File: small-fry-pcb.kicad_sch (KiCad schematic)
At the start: 139 parts, among them U1 Pico

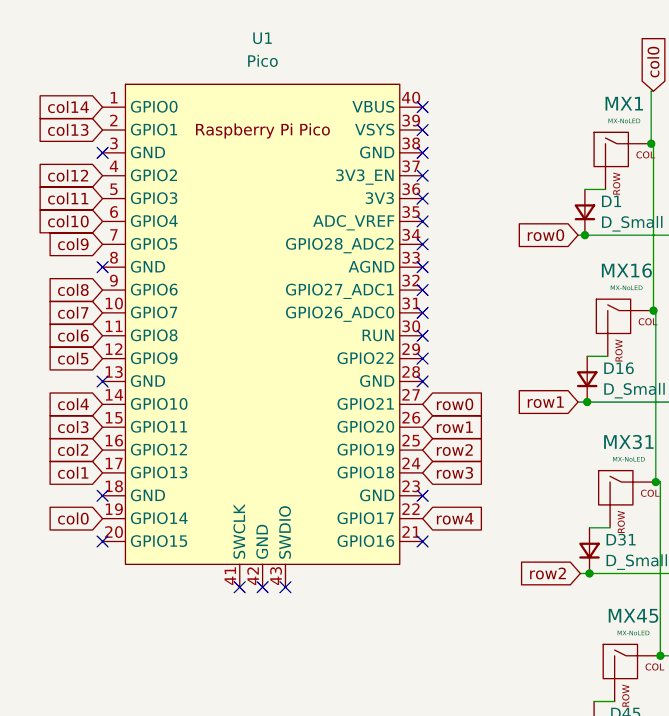
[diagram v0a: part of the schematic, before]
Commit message: Squashed commit of the following:
commit e493926800ae8eeeb9c8551a418d401659cc4f4a
Author: anchovie-codes <littlebrother.free@gmail.com>
Date:   Sun Nov 10 19:39:24 2024 -0500

    updated edge cuts and gerbers

commit a852bf54e9e750d94bc40db8a16316f7cdac5ac1
Author: anchovie-codes <littlebrother.free@gmail.com>
Date:   Sat Sep 28 17:49:30 2024 -0400

    fixed rows, generated gerbers

commit 9d77bf2fb49dd0b8cbfb8cfda25d822d23244967
Author: anchovie-codes <littlebrother.free@gmail.com>
Date:   Sat Sep 28 13:01:13 2024 -0400

    fixed cols

commit 5f5487953ddbebd1258b34876b9f208a7da505d8
Author: anchovie-codes <littlebrother.free@gmail.com>
Date:   Fri Sep 27 21:14:36 2024 -0400

    made it a fish
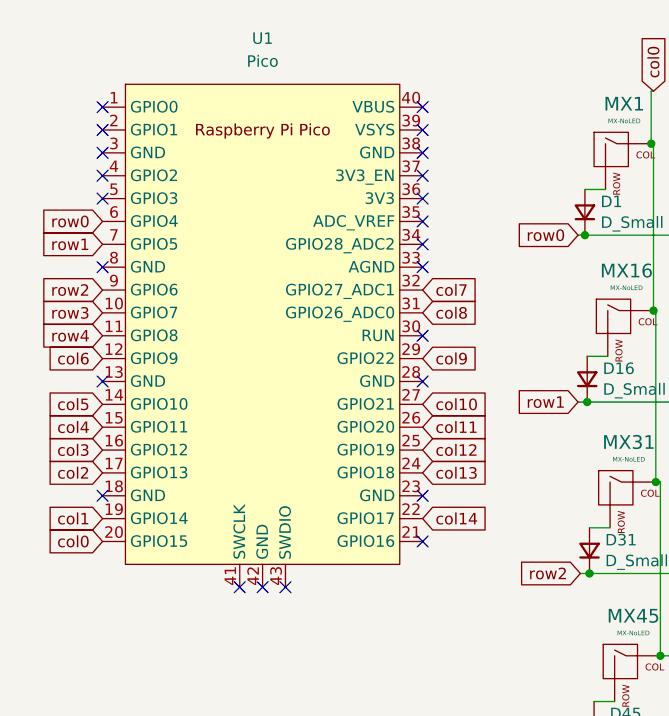
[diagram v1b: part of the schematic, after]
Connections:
- net col0: now also U1.20 (GPIO15); no longer U1.19 (GPIO14)
- net col1: now also U1.19 (GPIO14); no longer U1.17 (GPIO13)
- net col10: now also U1.27 (GPIO21); no longer U1.6 (GPIO4)
- net col11: now also U1.26 (GPIO20); no longer U1.5 (GPIO3)
- net col12: now also U1.25 (GPIO19); no longer U1.4 (GPIO2)
- net col13: now also U1.24 (GPIO18); no longer U1.2 (GPIO1)
- net col14: now also U1.22 (GPIO17); no longer U1.1 (GPIO0)
- net col2: now also U1.17 (GPIO13); no longer U1.16 (GPIO12)
- net col3: now also U1.16 (GPIO12); no longer U1.15 (GPIO11)
- net col4: now also U1.15 (GPIO11); no longer U1.14 (GPIO10)
- net col5: now also U1.14 (GPIO10); no longer U1.12 (GPIO9)
- net col6: now also U1.12 (GPIO9); no longer U1.11 (GPIO8)
- net col7: now also U1.32 (GPIO27_ADC1); no longer U1.10 (GPIO7)
- net col8: now also U1.31 (GPIO26_ADC0); no longer U1.9 (GPIO6)
- net col9: now also U1.29 (GPIO22); no longer U1.7 (GPIO5)
- net row0: now also U1.6 (GPIO4); no longer U1.27 (GPIO21)
- net row1: now also U1.7 (GPIO5); no longer U1.26 (GPIO20)
- net row2: now also U1.9 (GPIO6); no longer U1.25 (GPIO19)
- net row3: now also U1.10 (GPIO7); no longer U1.24 (GPIO18)
- net row4: now also U1.11 (GPIO8); no longer U1.22 (GPIO17)
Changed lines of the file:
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@@
 	)
 	(no_connect
+		(at 20.32 29.21)
+	)
+	(no_connect
 		(at 55.88 69.85)
 	)
@@
 	)
 	(no_connect
-		(at 55.88 41.91)
+		(at 20.32 26.67)
 	)
 	(no_connect
@@
 	)
 	(no_connect
-		(at 55.88 54.61)
+		(at 55.88 41.91)
 	)
 	(no_connect
-		(at 55.88 49.53)
+		(at 40.64 80.01)
 	)
 	(no_connect
-		(at 40.64 80.01)
+		(at 20.32 34.29)
 	)
 	(no_connect
@@
 	)
 	(no_connect
-		(at 20.32 74.93)
-	)
-	(no_connect
-		(at 55.88 46.99)
+		(at 20.32 36.83)
 	)
 	(no_connect
@@
 		)
 	)
-	(global_label "col14"
-		(shape input)
-		(at 20.32 26.67 180)
-		(fields_autoplaced yes)
-		(effects
-			(font
-				(size 1.27 1.27)
-			)
-			(justify right)
-		)
-		(property "Intersheetrefs" "${INTERSHEET_REFS}"
-			(at 12.6672 26.67 0)
-			(effects
-				(font
-					(size 1.27 1.27)
-				)
-				(justify right)
-				(hide yes)
-			)
-		)
-	)
-	(global_label "row0"
+	(global_label "col10"
 		(shape input)
 		(at 55.88 59.69 0)
@@
 		)
 		(property "Intersheetrefs" "${INTERSHEET_REFS}"
-			(at 62.6862 59.69 0)
+			(at 63.5328 59.69 0)
 			(effects
 				(font
@@
 		)
 	)
-	(global_label "col13"
+	(global_label "col5"
 		(shape input)
-		(at 20.32 29.21 180)
+		(at 20.32 59.69 180)
 		(fields_autoplaced yes)
 		(effects
@@
 		)
 		(property "Intersheetrefs" "${INTERSHEET_REFS}"
-			(at 12.6672 29.21 0)
+			(at 13.8767 59.69 0)
 			(effects
 				(font
@@
 		)
 	)
-	(global_label "col12"
+	(global_label "col1"
 		(shape input)
-		(at 20.32 34.29 180)
+		(at 20.32 72.39 180)
 		(fields_autoplaced yes)
 		(effects
@@
 		)
 		(property "Intersheetrefs" "${INTERSHEET_REFS}"
-			(at 12.6672 34.29 0)
+			(at 13.8767 72.39 0)
 			(effects
 				(font
@@
 		)
 	)
-	(global_label "col4"
+	(global_label "col2"
 		(shape input)
-		(at 20.32 59.69 180)
-		(fields_autoplaced yes)
+		(at 102.616 24.892 90)
 		(effects
 			(font
 				(size 1.27 1.27)
 			)
-			(justify right)
+			(justify left)
 		)
 		(property "Intersheetrefs" "${INTERSHEET_REFS}"
-			(at 13.8767 59.69 0)
+			(at 102.616 24.892 0)
 			(effects
 				(font
 					(size 1.27 1.27)
 				)
-				(justify right)
 				(hide yes)
 			)
 		)
 	)
-	(global_label "col0"
+	(global_label "col4"
 		(shape input)
-		(at 20.32 72.39 180)
+		(at 20.32 62.23 180)
 		(fields_autoplaced yes)
 		(effects
@@
 		)
 		(property "Intersheetrefs" "${INTERSHEET_REFS}"
-			(at 13.8767 72.39 0)
+			(at 13.8767 62.23 0)
 			(effects
 				(font
@@
 		)
 	)
-	(global_label "col2"
+	(global_label "col14"
 		(shape input)
-		(at 102.616 24.892 90)
+		(at 55.88 72.39 0)
+		(fields_autoplaced yes)
 		(effects
 			(font
@@
 		)
 		(property "Intersheetrefs" "${INTERSHEET_REFS}"
-			(at 102.616 24.892 0)
+			(at 63.5328 72.39 0)
 			(effects
 				(font
 					(size 1.27 1.27)
 				)
+				(justify left)
 				(hide yes)
 			)
@@
 	(global_label "col3"
 		(shape input)
-		(at 20.32 62.23 180)
+		(at 20.32 64.77 180)
 		(fields_autoplaced yes)
 		(effects
@@
 		)
 		(property "Intersheetrefs" "${INTERSHEET_REFS}"
-			(at 13.8767 62.23 0)
+			(at 13.8767 64.77 0)
 			(effects
 				(font
@@
 		)
 	)
-	(global_label "row4"
+	(global_label "col7"
 		(shape input)
-		(at 55.88 72.39 0)
+		(at 55.88 46.99 0)
 		(fields_autoplaced yes)
 		(effects
@@
 		)
 		(property "Intersheetrefs" "${INTERSHEET_REFS}"
-			(at 62.6862 72.39 0)
+			(at 62.3233 46.99 0)
 			(effects
 				(font
@@
 		)
 	)
-	(global_label "col2"
-		(shape input)
-		(at 20.32 64.77 180)
-		(fields_autoplaced yes)
-		(effects
-			(font
-				(size 1.27 1.27)
-			)
-			(justify right)
-		)
-		(property "Intersheetrefs" "${INTERSHEET_REFS}"
-			(at 13.8767 64.77 0)
-			(effects
-				(font
-					(size 1.27 1.27)
-				)
-				(justify right)
-				(hide yes)
-			)
-		)
-	)
 	(global_label "row0"
 		(shape input)
@@
 		)
 	)
-	(global_label "row2"
+	(global_label "col12"
 		(shape input)
 		(at 55.88 64.77 0)
@@
 		)
 		(property "Intersheetrefs" "${INTERSHEET_REFS}"
-			(at 62.6862 64.77 0)
+			(at 63.5328 64.77 0)
 			(effects
 				(font
@@
 		)
 	)
-	(global_label "col9"
+	(global_label "row1"
 		(shape input)
 		(at 20.32 41.91 180)
@@
 		)
 		(property "Intersheetrefs" "${INTERSHEET_REFS}"
-			(at 13.8767 41.91 0)
+			(at 13.5138 41.91 0)
 			(effects
 				(font
@@
 		)
 	)
-	(global_label "row3"
+	(global_label "col13"
 		(shape input)
 		(at 55.88 67.31 0)
@@
 		)
 		(property "Intersheetrefs" "${INTERSHEET_REFS}"
-			(at 62.6862 67.31 0)
+			(at 63.5328 67.31 0)
 			(effects
 				(font
@@
 		)
 	)
+	(global_label "row4"
+		(shape input)
+		(at 20.32 52.07 180)
+		(fields_autoplaced yes)
+		(effects
+			(font
+				(size 1.27 1.27)
+			)
+			(justify right)
+		)
+		(property "Intersheetrefs" "${INTERSHEET_REFS}"
+			(at 13.5138 52.07 0)
+			(effects
+				(font
+					(size 1.27 1.27)
+				)
+				(justify right)
+				(hide yes)
+			)
+		)
+	)
 	(global_label "row1"
 		(shape input)
@@
 		)
 	)
-	(global_label "col11"
+	(global_label "col8"
 		(shape input)
-		(at 20.32 36.83 180)
+		(at 55.88 49.53 0)
 		(fields_autoplaced yes)
 		(effects
@@
 				(size 1.27 1.27)
 			)
-			(justify right)
+			(justify left)
 		)
 		(property "Intersheetrefs" "${INTERSHEET_REFS}"
-			(at 12.6672 36.83 0)
+			(at 62.3233 49.53 0)
 			(effects
 				(font
 					(size 1.27 1.27)
 				)
-				(justify right)
+				(justify left)
 				(hide yes)
 			)
 		)
 	)
-	(global_label "col7"
+	(global_label "row3"
 		(shape input)
 		(at 20.32 49.53 180)
@@
 		)
 		(property "Intersheetrefs" "${INTERSHEET_REFS}"
-			(at 13.8767 49.53 0)
+			(at 13.5138 49.53 0)
 			(effects
 				(font
@@
 		)
 	)
-	(global_label "col10"
+	(global_label "row0"
 		(shape input)
 		(at 20.32 39.37 180)
@@
 		)
 		(property "Intersheetrefs" "${INTERSHEET_REFS}"
-			(at 12.6672 39.37 0)
+			(at 13.5138 39.37 0)
 			(effects
 				(font
@@
 		)
 	)
-	(global_label "col6"
+	(global_label "col0"
 		(shape input)
-		(at 20.32 52.07 180)
+		(at 20.32 74.93 180)
 		(fields_autoplaced yes)
 		(effects
@@
 		)
 		(property "Intersheetrefs" "${INTERSHEET_REFS}"
-			(at 13.8767 52.07 0)
+			(at 13.8767 74.93 0)
 			(effects
 				(font
@@
 		)
 	)
-	(global_label "col8"
+	(global_label "row2"
 		(shape input)
 		(at 20.32 46.99 180)
@@
 		)
 		(property "Intersheetrefs" "${INTERSHEET_REFS}"
-			(at 13.8767 46.99 0)
+			(at 13.5138 46.99 0)
 			(effects
 				(font
@@
 		)
 	)
-	(global_label "row1"
+	(global_label "col11"
 		(shape input)
 		(at 55.88 62.23 0)
@@
 		)
 		(property "Intersheetrefs" "${INTERSHEET_REFS}"
-			(at 62.6862 62.23 0)
+			(at 63.5328 62.23 0)
 			(effects
 				(font
@@
 		)
 	)
-	(global_label "col1"
+	(global_label "col9"
+		(shape input)
+		(at 55.88 54.61 0)
+		(fields_autoplaced yes)
+		(effects
+			(font
+				(size 1.27 1.27)
+			)
+			(justify left)
+		)
+		(property "Intersheetrefs" "${INTERSHEET_REFS}"
+			(at 62.3233 54.61 0)
+			(effects
+				(font
+					(size 1.27 1.27)
+				)
+				(justify left)
+				(hide yes)
+			)
+		)
+	)
+	(global_label "col2"
 		(shape input)
 		(at 20.32 67.31 180)
@@
 		)
 	)
-	(global_label "col5"
+	(global_label "col6"
 		(shape input)
 		(at 20.32 54.61 180)
